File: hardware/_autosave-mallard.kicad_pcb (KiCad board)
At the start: 4 copper layers, 101.6 x 101.1 mm, 87 parts, among them J1 USB_A, J2 Conn_02x03_Odd_Even, J3 Conn_01x03, J4 Conn_01x03, J5 Conn_01x03, J6 Conn_01x03, SW1 RESET Switch, U10 LM828, U11 STM32L4Q5xx, U12 LTC3529EDCB, U4 BQ24210DQCT, U5 TMUX1309, U6 TMUX1309, U7 LMP7721, U8 TPS71710DRVR, U9 LMV554

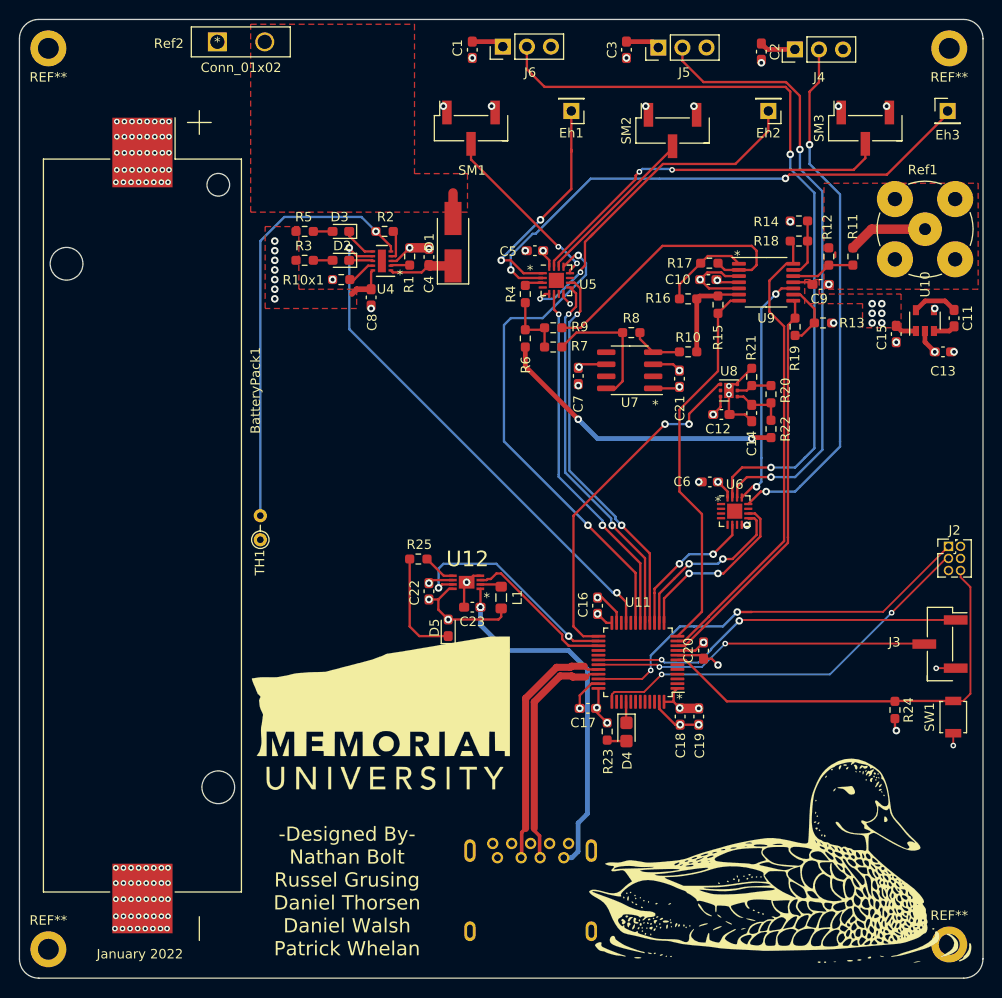
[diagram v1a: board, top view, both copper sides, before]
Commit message: STM32_USB_OTG_UPDATE_1
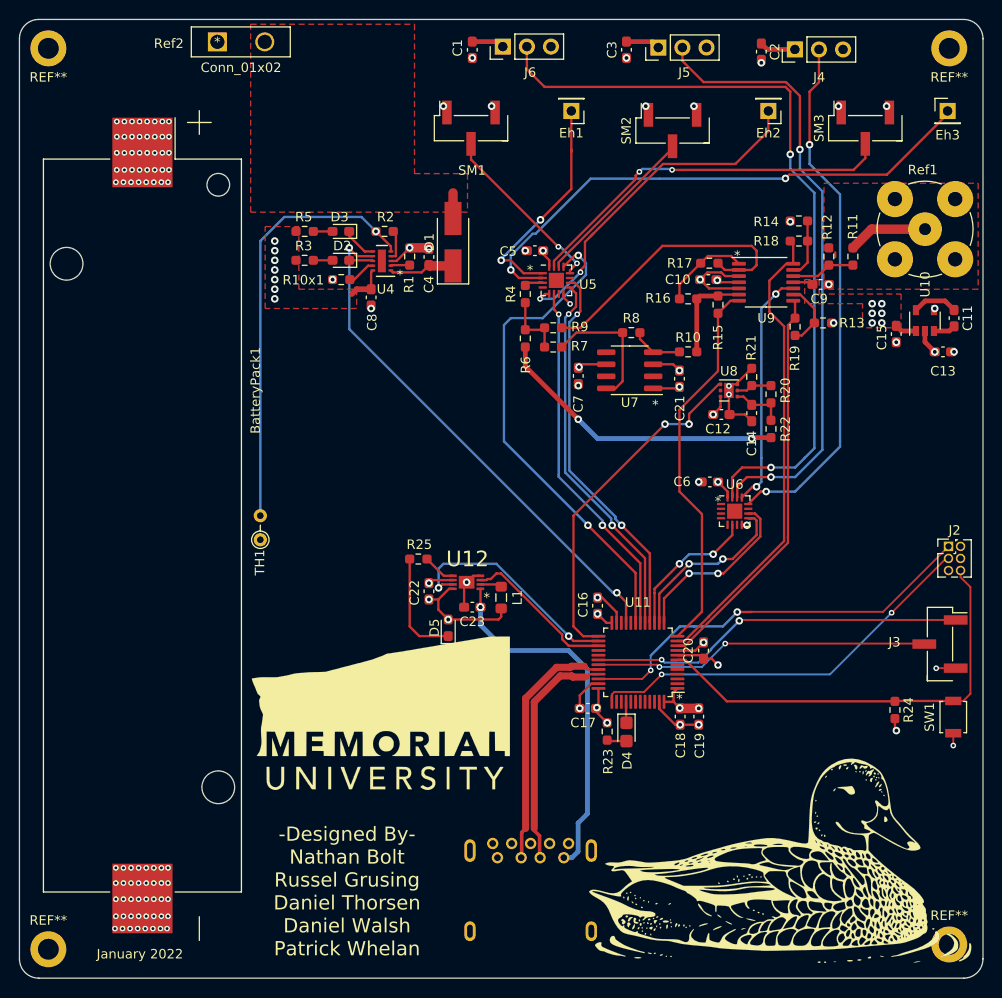
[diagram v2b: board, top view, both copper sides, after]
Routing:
- added copper zone on In2.Cu, net +3V3
- added copper zone on In2.Cu, net -3V3
- added copper zone on In1.Cu, net GND
- removed copper zone on Power, net +3V3
- removed copper zone on Power, net -3V3
- removed copper zone on GND, net GND
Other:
- net class Default removed
